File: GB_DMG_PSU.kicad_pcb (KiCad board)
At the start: 2 copper layers, 15 x 65 mm, 22 parts, among them J2 Conn_01x04, U1 R1283K001C-TR

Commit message: manufacturing files
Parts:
- C10, C7: value C -> as large as possible
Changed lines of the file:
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@@
 			(outputformat 1)
 			(mirror no)
-			(drillshape 1)
+			(drillshape 0)
 			(scaleselection 1)
-			(outputdirectory "")
+			(outputdirectory "gerber")
 		)
 	)
@@
 			)
 		)
-		(property "Value" "C"
+		(property "Value" "as large as possible"
 			(at 0 2.35 90)
 			(layer "F.Fab")
@@
 			)
 		)
-		(property "Value" "C"
+		(property "Value" "as large as possible"
 			(at 0 2.35 270)
 			(layer "F.Fab")

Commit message: don't need backups online
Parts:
- C6: value 47pF -> 330pF
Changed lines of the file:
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@@
 			)
 		)
-		(property "Value" "47pF"
+		(property "Value" "330pF"
 			(at 0 1.43 90)
 			(layer "F.Fab")

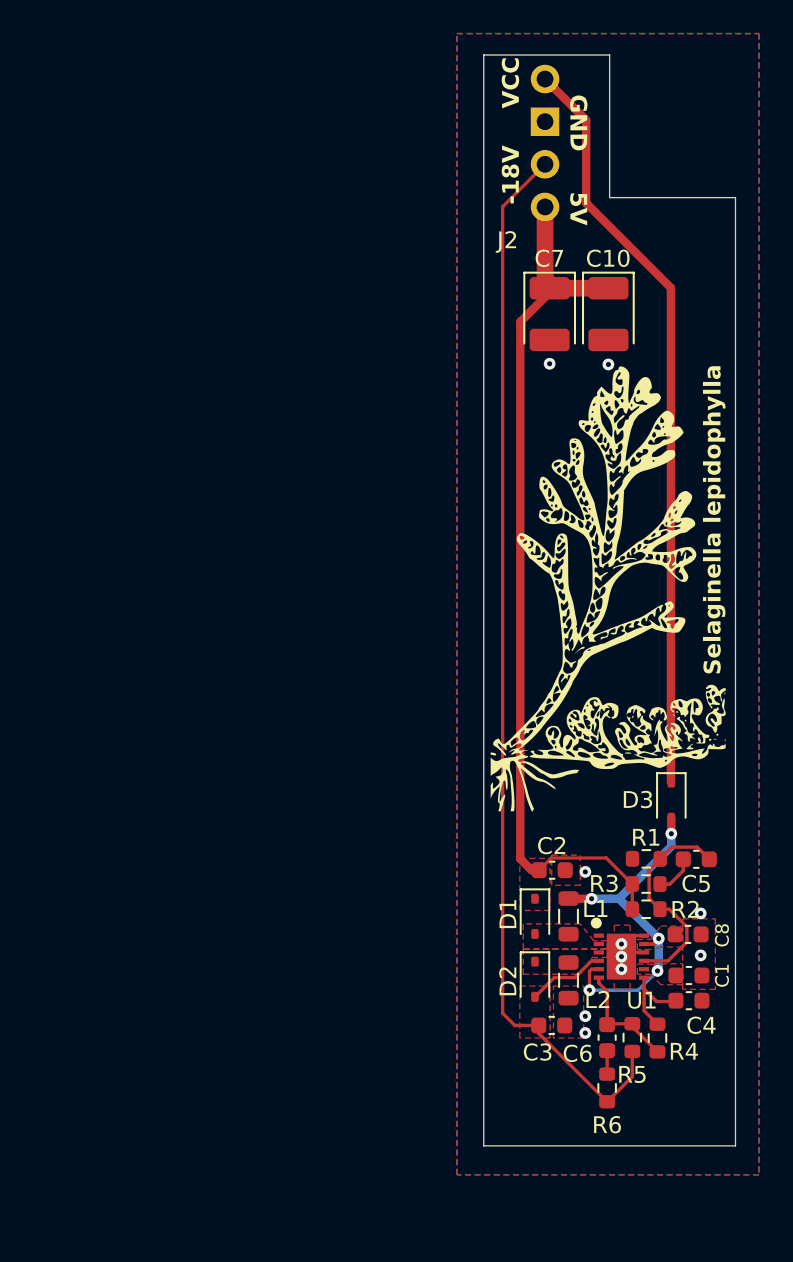
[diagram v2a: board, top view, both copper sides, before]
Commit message: V2
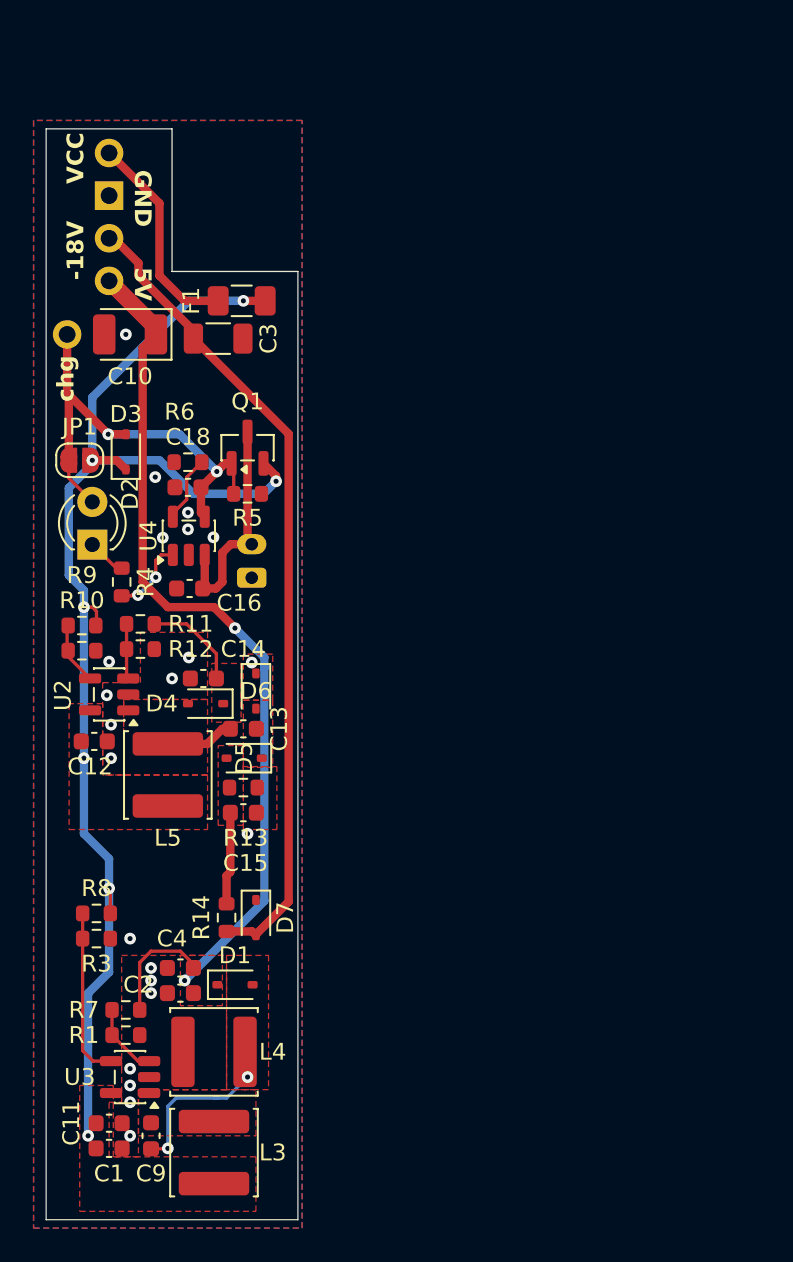
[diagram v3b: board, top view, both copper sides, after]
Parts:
- removed C5: 68pF, Capacitor_SMD:C_0603_1608Metric
- removed C6: 330pF, Capacitor_SMD:C_0603_1608Metric
- removed C7: as large as possible, Capacitor_Tantalum_SMD:CP_EIA-3528-12_Kemet-T
- removed C8: 4,7µF, Capacitor_SMD:C_0603_1608Metric
- removed L1, L2: 4,7µH, Inductor_SMD:L_0805_2012Metric
- removed R2: 42k, Resistor_SMD:R_0603_1608Metric
- removed U1: R1283K001C-TR, footprints:PE-DFNPL2730-12-180404_NMD
- added C11: 10µF, Capacitor_SMD:C_0603_1608Metric, F.Cu at (73.2, 85.0)
- added C12: 10µF, Capacitor_SMD:C_0603_1608Metric, F.Cu at (72.4, 62.2)
- added C13: 1µF, Capacitor_SMD:C_0603_1608Metric, F.Cu at (81.2, 61.5)
- added C14: 10µF, Capacitor_SMD:C_0603_1608Metric, F.Cu at (78.9, 58.5)
- added C15: 1µF, Capacitor_SMD:C_0603_1608Metric, F.Cu at (81.2, 66.5)
- added C16: 10uF, Capacitor_SMD:C_0603_1608Metric, F.Cu at (78.0, 53.1)
- added C18: 100nF, Capacitor_SMD:C_0603_1608Metric, F.Cu at (78.0, 47.1)
- added C9: 1µF, Capacitor_SMD:C_0603_1608Metric, F.Cu at (75.8, 85.8)
- added D4: D, Diode_SMD:D_SOD-323, F.Cu at (79.0, 60.0)
- added D5: D, Diode_SMD:D_SOD-323, F.Cu at (81.3, 63.2)
- added D6: D, Diode_SMD:D_SOD-323, F.Cu at (82.0, 59.2)
- added D7: 18V, Diode_SMD:D_SOD-323, F.Cu at (82.0, 72.8)
- added F1: Fuse, Fuse:Fuse_1206_3216Metric, F.Cu at (81.2, 36.0)
- added J3: Conn_01x02, Connector_JST:JST_PH_S2B-PH-K_1x02_P2.00mm_Horizontal, B.Cu at (81.8, 52.5)
- added J4: Conn_01x01, Connector_PinHeader_2.54mm:PinHeader_1x01_P2.54mm_Vertical, F.Cu at (70.8, 38.0)
- added JP1: Jumper, Jumper:SolderJumper-2_P1.3mm_Open_RoundedPad1.0x1.5mm, F.Cu at (71.5, 45.5)
- added L3: 10µH, Inductor_SMD:L_APV_ANR5040, F.Cu at (79.5, 86.8)
- added L4: 10µH, Inductor_SMD:L_APV_ANR5040, F.Cu at (79.5, 80.8)
- added L5: 10µH, Inductor_SMD:L_APV_ANR5040, F.Cu at (76.8, 64.2)
- added Q1: BSS84, Package_TO_SOT_SMD:SOT-23, F.Cu at (81.5, 44.8)
- added R10: 100k, Resistor_SMD:R_0603_1608Metric, F.Cu at (71.6, 56.8)
- added R11: 100k, Resistor_SMD:R_0603_1608Metric, F.Cu at (75.1, 55.2)
- added R12: 6,8k, Resistor_SMD:R_0603_1608Metric, F.Cu at (75.1, 56.8)
- added R13: 15k, Resistor_SMD:R_0603_1608Metric, F.Cu at (81.2, 65.0)
- added R14: TBD, Resistor_SMD:R_0603_1608Metric, F.Cu at (80.2, 72.8)
- added R7: 100k, Resistor_SMD:R_0603_1608Metric, F.Cu at (74.2, 78.2)
- added R8: 100k, Resistor_SMD:R_0603_1608Metric, F.Cu at (72.5, 72.5)
- added R9: 100k, Resistor_SMD:R_0603_1608Metric, F.Cu at (71.6, 55.3)
- added U2: LGS6302B5, Package_TO_SOT_SMD:SOT-23-5, F.Cu at (73.3, 59.5)
- added U3: LGS6302B5, Package_TO_SOT_SMD:SOT-23-5, F.Cu at (74.5, 82.2)
- added U4: MCP73831, Package_TO_SOT_SMD:SOT-23-5, F.Cu at (78.0, 50.0)
- C1: value 4,7µF -> 10µF
- C3: footprint Capacitor_SMD:C_0603_1608Metric -> Capacitor_SMD:C_1206_3216Metric
- C4: value 100nF -> 10µF
- D2: value D -> LED_CHR; footprint Diode_SMD:D_SOD-323 -> LED_THT:LED_D3.0mm
- R1: value 10k -> 33k
- R3: value 1k -> 100k
- R4: value 6,8k -> 1K
- R5: value 100k -> 100K
- R6: value 1k -> 2K
- moved C3 45.5 mm to (79.8, 38.2)
- moved R6 44.9 mm to (78.0, 45.6), turned to 0 degrees
- moved R4 41.9 mm to (74.0, 52.8), turned to -90 degrees
- moved R5 39.7 mm to (81.5, 47.5), turned to 180 degrees
- moved D3 38.6 mm to (74.2, 45.0), turned to 90 degrees
- moved D2 37.0 mm to (72.2, 50.5), turned to 90 degrees
- moved C1 36.1 mm to (73.2, 86.5)
- moved R3 32.9 mm to (72.5, 74.0)
- moved R1 32.7 mm to (74.2, 79.8), turned to 0 degrees
- moved C4 30.4 mm to (77.5, 75.8), turned to 180 degrees
- moved C10 28.5 mm to (74.5, 38.0), turned to 180 degrees
- moved J2 26.3 mm to (73.2, 34.8)
- moved C2 23.3 mm to (77.5, 77.2), turned to 180 degrees
- moved D1 18.3 mm to (80.8, 76.8), turned to 0 degrees
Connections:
- C3 pad 1: -VDC -> -18V
- C4 pad 1: VREF -> +5V
- D1 pad 2: /buck+ -> /sw2
- D2 pad 1: /buck- -> Net-(D2-K)
- D2 pad 2: -VDC -> VIN
- D3 pad 1: Net-(D3-K) -> VCC
- D3 pad 2: VCC -> VIN
- J2 pad 2: -VDC -> -18V
- J2 pad 4: Net-(D3-K) -> Net-(J2-Pin_4)
- R1 pad 1: FB1 -> Net-(U3-FB)
- R3 pad 1: +5V -> Net-(U3-EN)
- R3 pad 2: Net-(C5-Pad1) -> GND
- R4 pad 1: FB2 -> Net-(D2-K)
- R4 pad 2: VREF -> Net-(U4-STAT)
- R5 pad 1: -VDC -> GND
- R5 pad 2: FB2 -> VIN
- R6 pad 1: -VDC -> GND
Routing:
- net -VDC: track 68.6 -> 0.00 mm
- net VCC: track 21.7 -> 77.5 mm, vias 5 -> 7
- net -18V: track 0.00 -> 48.8 mm
- net Net-(D3-K): track 45.0 -> 0.00 mm
- net VIN: track 0.00 -> 28.5 mm, vias 0 -> 2
- net VBAT: track 0.00 -> 13.9 mm
- net FB1: track 13.0 -> 0.00 mm
- net Net-(J2-Pin_4): track 0.00 -> 12.7 mm
- net Net-(U3-EN): track 0.00 -> 10.4 mm
- net /sw2: track 0.00 -> 9.49 mm, vias 0 -> 2
- net FB2: track 6.82 -> 0.00 mm
- net +18V: track 0.00 -> 5.91 mm
- net VREF: track 5.27 -> 0.00 mm
- net /pump2: track 0.00 -> 5.02 mm
- net Net-(U4-STAT): track 0.00 -> 4.65 mm, vias 0 -> 2
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- added copper zone on F.Cu, net +18V
- added copper zone on F.Cu, net /pump1
- added copper zone on F.Cu, net /pump2
- added copper zone on F.Cu, net /sw
- added copper zone on F.Cu, net /sw2
- added copper zone on F.Cu, net /sw3
- removed copper zone on F.Cu, net -VDC
- removed copper zone on F.Cu, net /buck+
- removed copper zone on F.Cu, net /buck-
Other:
- board text added: "+ -"
- board text added: "chg"
